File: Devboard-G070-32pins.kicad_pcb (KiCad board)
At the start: 2 copper layers, 88.3 x 44 mm, 28 parts, among them J1 Conn_01x05, J2 Conn_01x07, J3 Conn_01x01, J4 Conn_01x07, J5 HW-769, J6 NS6312, J7 Conn_01x03, Q1 2N7002H, SW1 SW_MEC_5E, SW3 SW_MEC_5E, U2 STM32G070KBTx

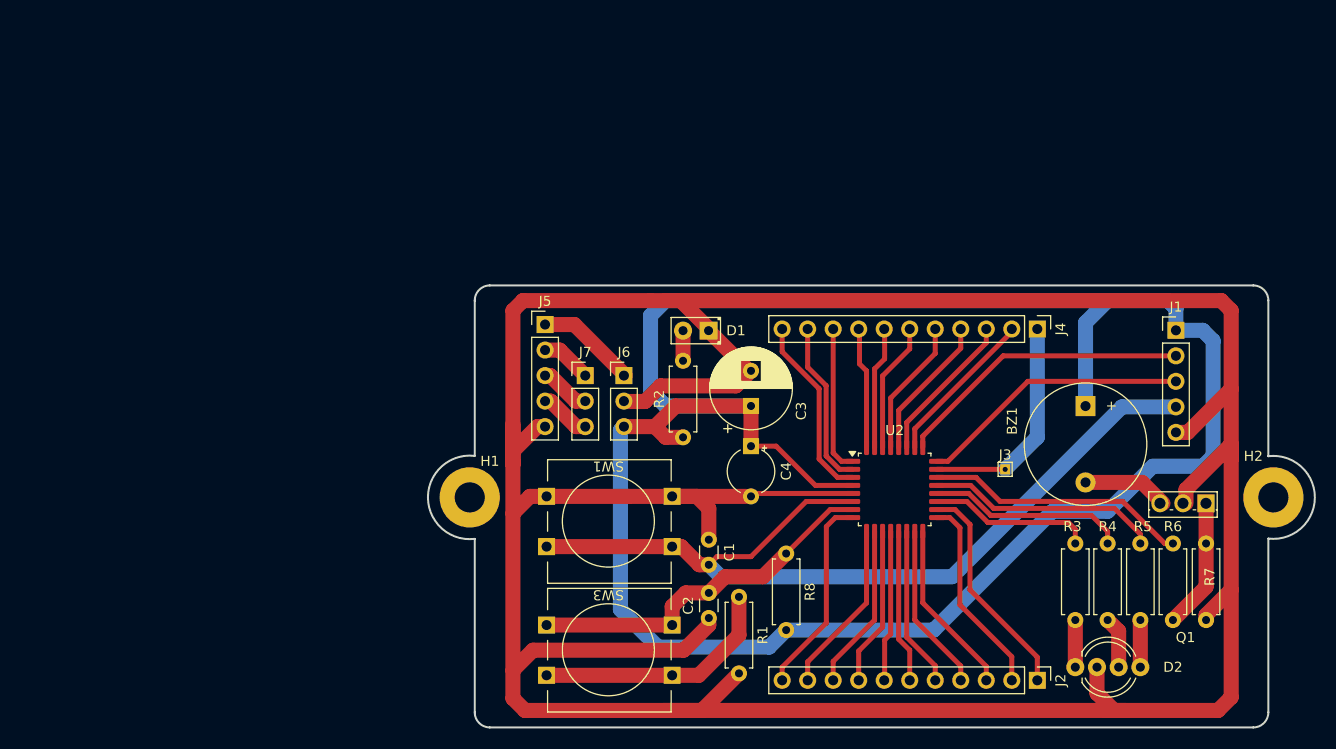
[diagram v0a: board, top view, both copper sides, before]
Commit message: perf: 45° micro
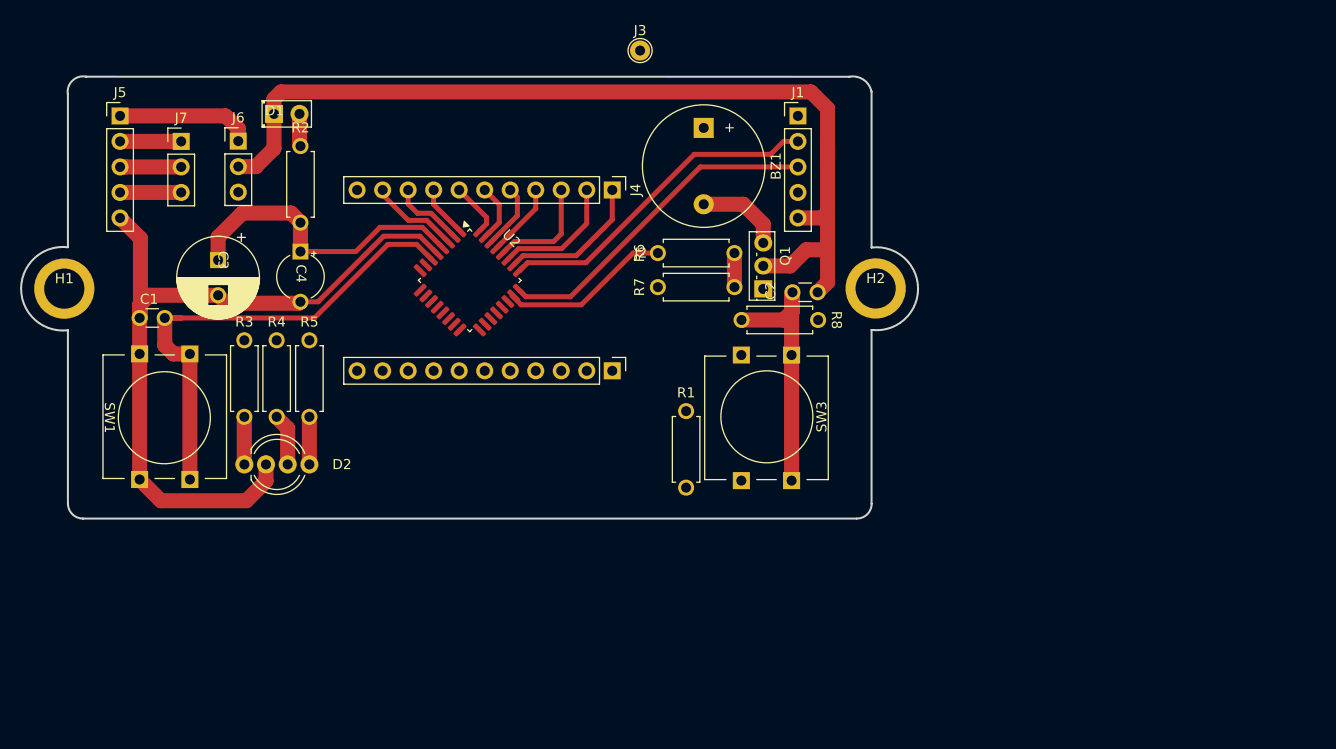
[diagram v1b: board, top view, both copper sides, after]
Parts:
- C1, C2: footprint Capacitor_THT:C_Disc_D3.0mm_W1.6mm_P2.50mm -> personalized:C_Disc_D1mm
- C3: footprint Capacitor_THT:CP_Radial_D8.0mm_P3.50mm -> personalized:CP_Radial_1mm
- C4: footprint Capacitor_THT:CP_Radial_Tantal_D4.5mm_P5.00mm -> personalized:CP_Radial_Tantal_1mm
- D1: footprint LED_THT:LED_D2.0mm_W4.8mm_H2.5mm_FlatTop -> personalized:LED_1mm
- H1, H2: footprint MountingHole:MountingHole_3mm_Pad -> personalized:V_1mm
- J3: footprint TestPoint:TestPoint_THTPad_1.0x1.0mm_Drill0.5mm -> TestPoint:TestPoint_THTPad_D2.0mm_Drill1.0mm
- R1, R2, R3, R4, R5, R6, R7, R8: footprint Resistor_THT:R_Axial_DIN0207_L6.3mm_D2.5mm_P7.62mm_Horizontal -> personalized:Resistor_THT_Horizontal_1mm
- moved D2 85.1 mm to (-19.2, 18.3)
- moved R3 85.1 mm to (-22.4, 13.6)
- moved R4 85.1 mm to (-19.2, 13.6)
- moved R5 85.1 mm to (-16.0, 13.6)
- moved C1 60.7 mm to (-32.7, 3.66), turned to 0 degrees
- moved R6 56.9 mm to (26.4, -2.72), turned to 180 degrees
- moved J3 55.3 mm to (17.0, -22.9)
- moved C3 55.0 mm to (-25.1, -2.02), turned to -90 degrees
- moved R7 53.4 mm to (26.4, 0.67), turned to 180 degrees
- moved J2 52.3 mm to (14.2, 9.00)
- moved SW1 50.3 mm to (-36.4, 13.7), turned to -90 degrees
- moved Q1 49.0 mm to (29.2, 0.85), turned to 90 degrees
- moved C4 48.9 mm to (-16.9, -2.87)
- moved D1 48.2 mm to (-19.4, -16.4), turned to 0 degrees
- moved U2 47.1 mm to (0.00, 0.00), turned to -45 degrees
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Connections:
- J2 pad 11: PA1 -> PA9
- J4 pad 1: PA12 -> PA15
- J4 pad 10: PC14 -> PC15
- J4 pad 11: PC15 -> PA1
- J4 pad 2: PA15 -> PB3
- J4 pad 3: PB3 -> PB4
- J4 pad 4: PB4 -> PB5
- J4 pad 5: PB5 -> PB6
- J4 pad 6: PB6 -> PB7
- J4 pad 7: PB7 -> PB8
- J4 pad 8: PB8 -> PB9
- J4 pad 9: PB9 -> PC14
- U2 pad 19: LED_R -> PA9
- U2 pad 21: LED_B -> LED_R
- U2 pad 22: Buzzer -> LED_B
- U2 pad 23: PA12 -> Buzzer
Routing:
- net +3V3: track 219.3 -> 30.6 mm
- net GND: track 355.5 -> 172.4 mm
- net NRST: track 87.8 -> 49.4 mm
- net Net-(R1-Pad1): track 24.6 -> 0.00 mm
- net LED_B: track 23.2 -> 0.00 mm
- net PA12: track 22.8 -> 0.00 mm
- net PA8: track 22.2 -> 0.00 mm
- net PB2: track 20.8 -> 0.00 mm
- net PA1: track 20.1 -> 0.00 mm
- net LED_G: track 20.0 -> 0.17 mm
- net PB1: track 17.4 -> 0.00 mm
- net PA2: track 17.3 -> 0.00 mm
- net PB0: track 16.7 -> 0.00 mm
- net PA3: track 16.5 -> 0.00 mm
- net PA4: track 16.4 -> 0.00 mm
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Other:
- board size 88.3 x 44 mm -> 89.3 x 44 mm

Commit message: board v1
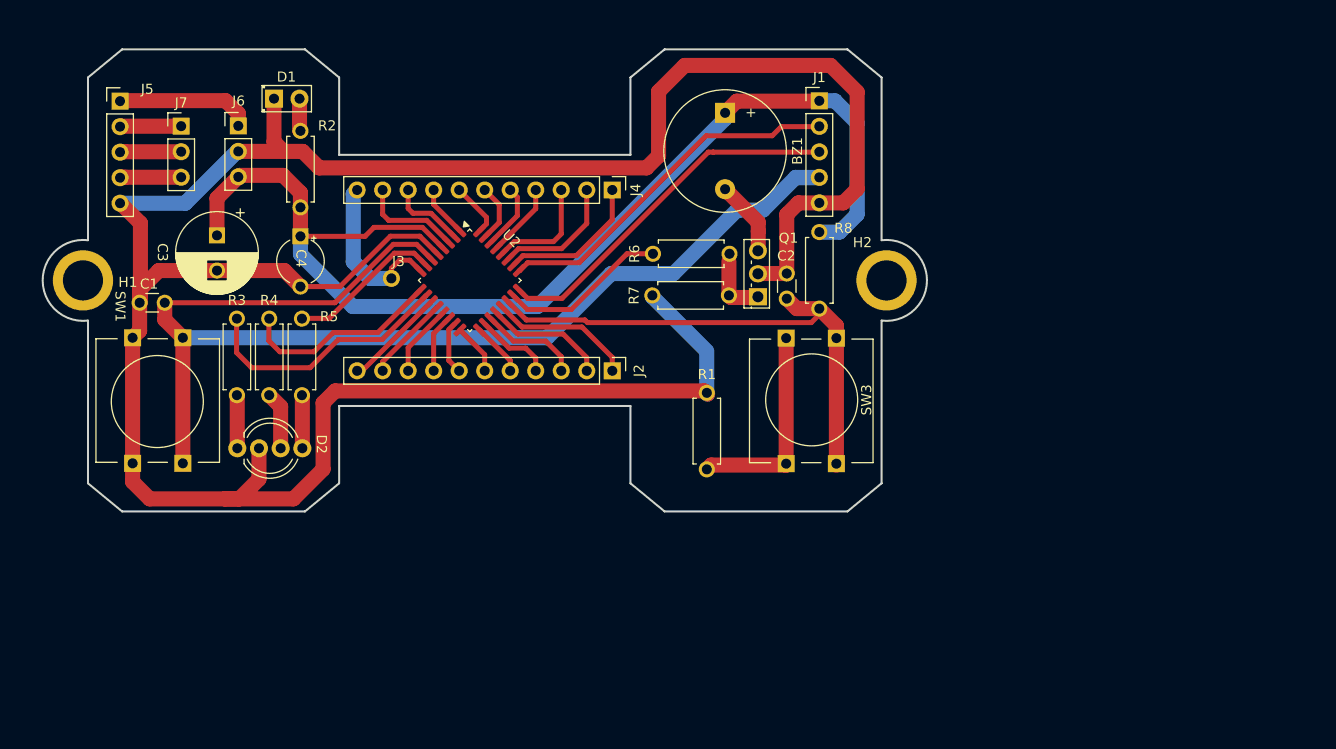
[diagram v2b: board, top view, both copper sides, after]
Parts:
- J3: footprint TestPoint:TestPoint_THTPad_D2.0mm_Drill1.0mm -> personalized:hole
- moved J3 33.6 mm to (-7.80, -0.20)
- moved R8 7.86 mm to (34.8, 2.86), turned to 90 degrees
- moved SW3 4.77 mm to (40.0, 11.9)
- moved C2 3.40 mm to (31.6, -0.56), turned to -90 degrees
- moved R1 2.75 mm to (23.6, 18.9)
- moved BZ1 2.61 mm to (25.4, -16.7)
- moved J1 2.61 mm to (34.8, -17.9)
- moved C3 2.46 mm to (-25.2, -4.48)
- moved R4 2.28 mm to (-20.0, 11.5)
- moved R5 2.28 mm to (-16.7, 11.5)
- moved R3 2.28 mm to (-23.2, 11.5)
- moved H1 2.03 mm to (-38.5, -0.50)
- moved SW1 1.76 mm to (-37.1, 12.1)
- moved D2 1.76 mm to (-19.9, 16.7)
- moved J6 1.52 mm to (-23.0, -15.4)
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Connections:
- J2 pad 1: PA8 -> PA10
- J2 pad 10: PA2 -> PA5
- J2 pad 11: PA9 -> PA4
- J2 pad 2: PB2 -> PC6
- J2 pad 3: PB1 -> PA9
- J2 pad 4: PB0 -> PA8
- J2 pad 5: PA7 -> PB2
- J2 pad 6: PA6 -> PB1
- J2 pad 7: PA5 -> PB0
- J2 pad 8: PA4 -> PA7
- J2 pad 9: PA3 -> PA6
- J3 pad 1: PA12 -> PA1
- U2 pad 10: PA3 -> LED_R
- U2 pad 20: LED_G -> PC6
- U2 pad 21: LED_R -> PA10
- U2 pad 22: LED_B -> BTN_Code
- U2 pad 7: BTN_Code -> LED_B
- U2 pad 9: PA2 -> LED_G
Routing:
- net GND: track 172.4 -> 265.9 mm
- net +3V3: track 30.6 -> 116.1 mm
- net NRST: track 49.4 -> 118.0 mm
- net BTN_Code: track 26.0 -> 52.7 mm
- net LED_R: track 0.06 -> 26.0 mm
- net Net-(R1-Pad1): track 0.00 -> 20.6 mm
- net LED_G: track 0.17 -> 20.6 mm
- net PA1: track 0.00 -> 16.4 mm
- net LED_B: track 0.00 -> 14.8 mm
- net PA10: track 0.00 -> 14.4 mm
- net PC6: track 0.00 -> 12.1 mm
- net PA4: track 0.00 -> 10.3 mm
- net PA9: track 0.00 -> 9.99 mm
- net PA5: track 0.00 -> 8.58 mm
- net PA8: track 0.00 -> 7.69 mm
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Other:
- board size 89.3 x 44 mm -> 88 x 46 mm
